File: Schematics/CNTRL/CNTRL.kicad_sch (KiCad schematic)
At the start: 129 parts, among them J1 SWD, J10 Y+, J11 Y-, J12 693071020811, J13 3.3V, J14 NAVIG I2C, J15 I2C, J16 USART, J17 PYRO1_OSTTE020104, J18 PYRO3_OSTTE020104, J19 USB_A_TE_292303-7_Horizontal, J2 CONSMA001-SMD-G-T, J20 PYRO2_OSTTE020104, J21 PYRO4_OSTTE020104, J22 Reset Jumper, J3 3S LiPo, J4 F4, J5 F3, J6 F2, J7 F1, J8 X+, J9 X-, Q1 BUK9832-55A_CUX, Q2 BUK9832-55A_CUX, Q3 BUK9832-55A_CUX, Q4 BUK9832-55A_CUX, Q5 BUK9832-55A_CUX, SW1 Omron_B3F-10xx, SW2 Omron_B3F-10xx, U1 STM32405RGT6, U2 RFM95W-915S2, U3 TPS2117DRLR, U4 TPS563200, U5 AMS1117-3.3, U7 W25Q128JVSIQ, U8 USBLC6-2SC6, Y1 12MHz_ECS-120-18-33-JGN-TR3, Y2 32.768KHz_SC32S-7PF20PPM

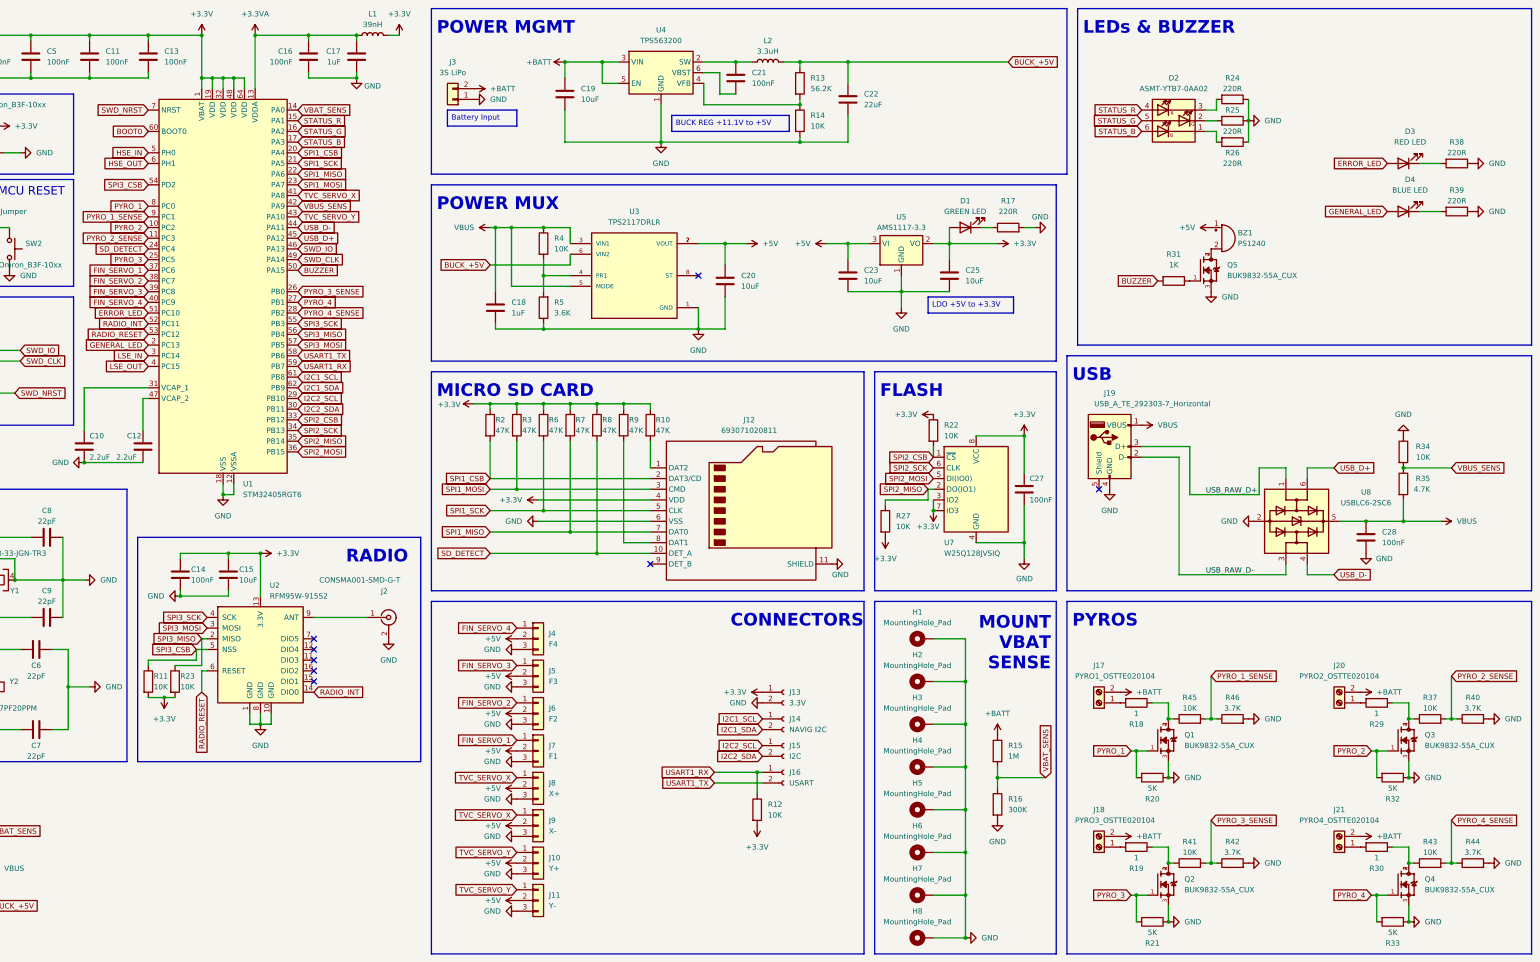
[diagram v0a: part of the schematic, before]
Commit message: CNTRL v1.1 fixes
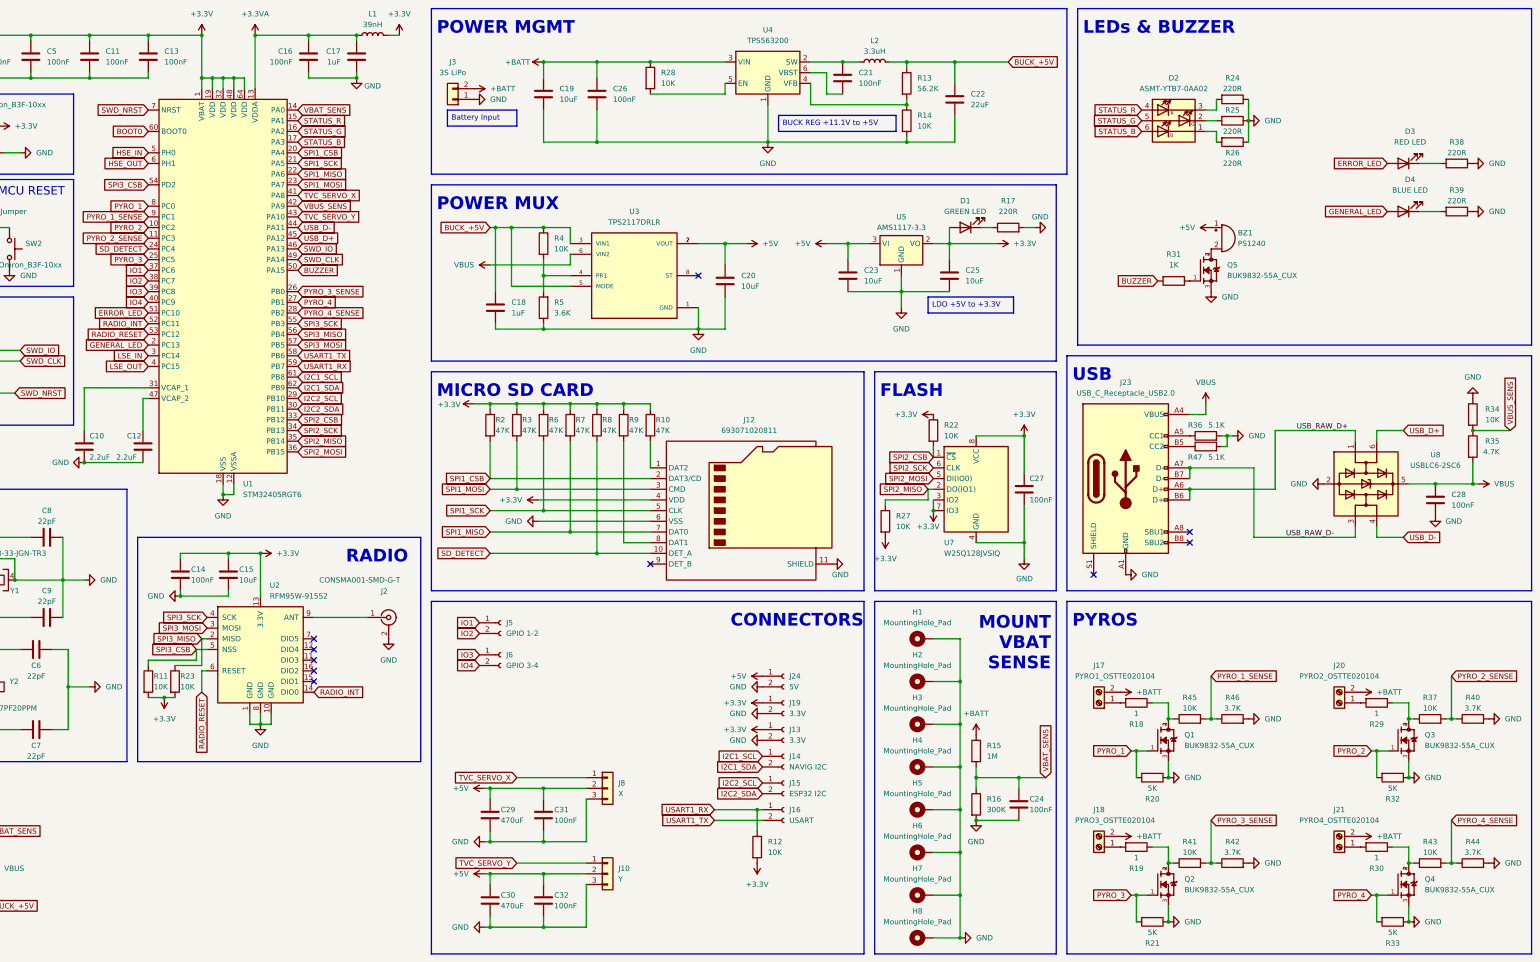
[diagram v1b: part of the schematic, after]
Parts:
- removed J11: Y-, Connector_PinHeader_2.54mm:PinHeader_1x03_P2.54mm_Vertical, symbol Connector_Generic:Conn_01x03
- removed J19: USB_A_TE_292303-7_Horizontal, Connector_USB:USB_A_TE_292303-7_Horizontal, symbol Connector:USB_A
- removed J4: F4, Connector_PinHeader_2.54mm:PinHeader_1x03_P2.54mm_Vertical, symbol Connector_Generic:Conn_01x03
- removed J5: F3, Connector_PinHeader_2.54mm:PinHeader_1x03_P2.54mm_Vertical, symbol Connector_Generic:Conn_01x03
- removed J6: F2, Connector_PinHeader_2.54mm:PinHeader_1x03_P2.54mm_Vertical, symbol Connector_Generic:Conn_01x03
- removed J7: F1, Connector_PinHeader_2.54mm:PinHeader_1x03_P2.54mm_Vertical, symbol Connector_Generic:Conn_01x03
- removed J9: X-, Connector_PinHeader_2.54mm:PinHeader_1x03_P2.54mm_Vertical, symbol Connector_Generic:Conn_01x03
- added C24, C26, C31, C32: 100nF, Capacitor_SMD:C_0603_1608Metric, symbol Device:C
- added C29, C30: 470uF, Capacitor_THT:CP_Radial_D6.3mm_P2.50mm, symbol Device:C
- added J19: 3.3V, Connector_JST:JST_XH_B2B-XH-A_1x02_P2.50mm_Vertical, symbol Connector:Conn_01x02_Socket
- added J23: USB_C_Receptacle_USB2.0, Connector_USB:USB_C_Receptacle_GCT_USB4105-xx-A_16P_TopMnt_Horizontal, symbol Connector:USB_C_Receptacle_USB2.0
- added J24: 5V, Connector_JST:JST_XH_B2B-XH-A_1x02_P2.50mm_Vertical, symbol Connector:Conn_01x02_Socket
- added J5: GPIO 1-2, TerminalBlock_Phoenix:TerminalBlock_Phoenix_MPT-0,5-2-2.54_1x02_P2.54mm_Horizontal, symbol Connector:Conn_01x02_Socket
- added J6: GPIO 3-4, TerminalBlock_Phoenix:TerminalBlock_Phoenix_MPT-0,5-2-2.54_1x02_P2.54mm_Horizontal, symbol Connector:Conn_01x02_Socket
- added R28: 10K, Resistor_SMD:R_0603_1608Metric, symbol Device:R
- added R36, R47: 5.1K, Resistor_SMD:R_0603_1608Metric, symbol Device:R
- J10: value Y+ -> Y; footprint Connector_PinHeader_2.54mm:PinHeader_1x03_P2.54mm_Vertical -> TerminalBlock_Phoenix:TerminalBlock_Phoenix_MPT-0,5-3-2.54_1x03_P2.54mm_Horizontal
- J15: value I2C -> ESP32 I2C
- J8: value X+ -> X; footprint Connector_PinHeader_2.54mm:PinHeader_1x03_P2.54mm_Vertical -> TerminalBlock_Phoenix:TerminalBlock_Phoenix_MPT-0,5-3-2.54_1x03_P2.54mm_Horizontal
- Q1, Q2, Q3, Q4, Q5: footprint BUK9832-55A_CUX:TRANS_BUK9832-55A_CUX -> External:TRANS_BUK9832-55A_CUX
- U7: footprint Package_SO:SOIC-8_5.23x5.23mm_P1.27mm -> Package_SO:SOIC-8_5.3x5.3mm_P1.27mm
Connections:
- net +3.3V: now also J19.1 (Pin_1)
- net +5V: now also C29.2, C30.2, C31.2, C32.2, J24.1 (Pin_1)
- net +BATT: now also C26.1, R28.1; no longer U4.5 (EN)
- net BUCK_+5V: now also C18.1, R4.1, U3.3 (VIN1), U3.5 (MODE); no longer U3.6 (VIN2)
- net GND: now also C24.1, C26.2, C29.1, C30.1, C31.1, C32.1, J19.2 (Pin_2), J23.A1 (GND), J23.A12 (GND), J23.B1 (GND), J23.B12 (GND), J24.2 (Pin_2), R36.2, R47.2
- net USB_RAW_D+: now also J23.A6 (D+), J23.B6 (D+)
- net USB_RAW_D-: now also J23.A7 (D-), J23.B7 (D-)
- net VBAT_SENS: now also C24.2
- net VBUS: now also U3.6 (VIN2), J23.A4 (VBUS), J23.A9 (VBUS), J23.B4 (VBUS), J23.B9 (VBUS); no longer C18.1, R4.1, U3.3 (VIN1), U3.5 (MODE)
- net FIN_SERVO_1 renamed IO1
- net IO1: now also J5.1 (Pin_1)
- net FIN_SERVO_2 renamed IO2
- net IO2: now also J5.2 (Pin_2)
- net FIN_SERVO_3 renamed IO3
- net IO3: now also J6.1 (Pin_1)
- net FIN_SERVO_4 renamed IO4
- net IO4: now also J6.2 (Pin_2)
- new net: R28.2, U4.5 (EN)
- new net: J23.B5 (CC2), R47.1
- new net: J23.A5 (CC1), R36.1
- no-connect marks 10 -> 12
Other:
- moved on the sheet: C19, C21, C22, C28, J10, J13, J14, J15, J16, J8, L2, R12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

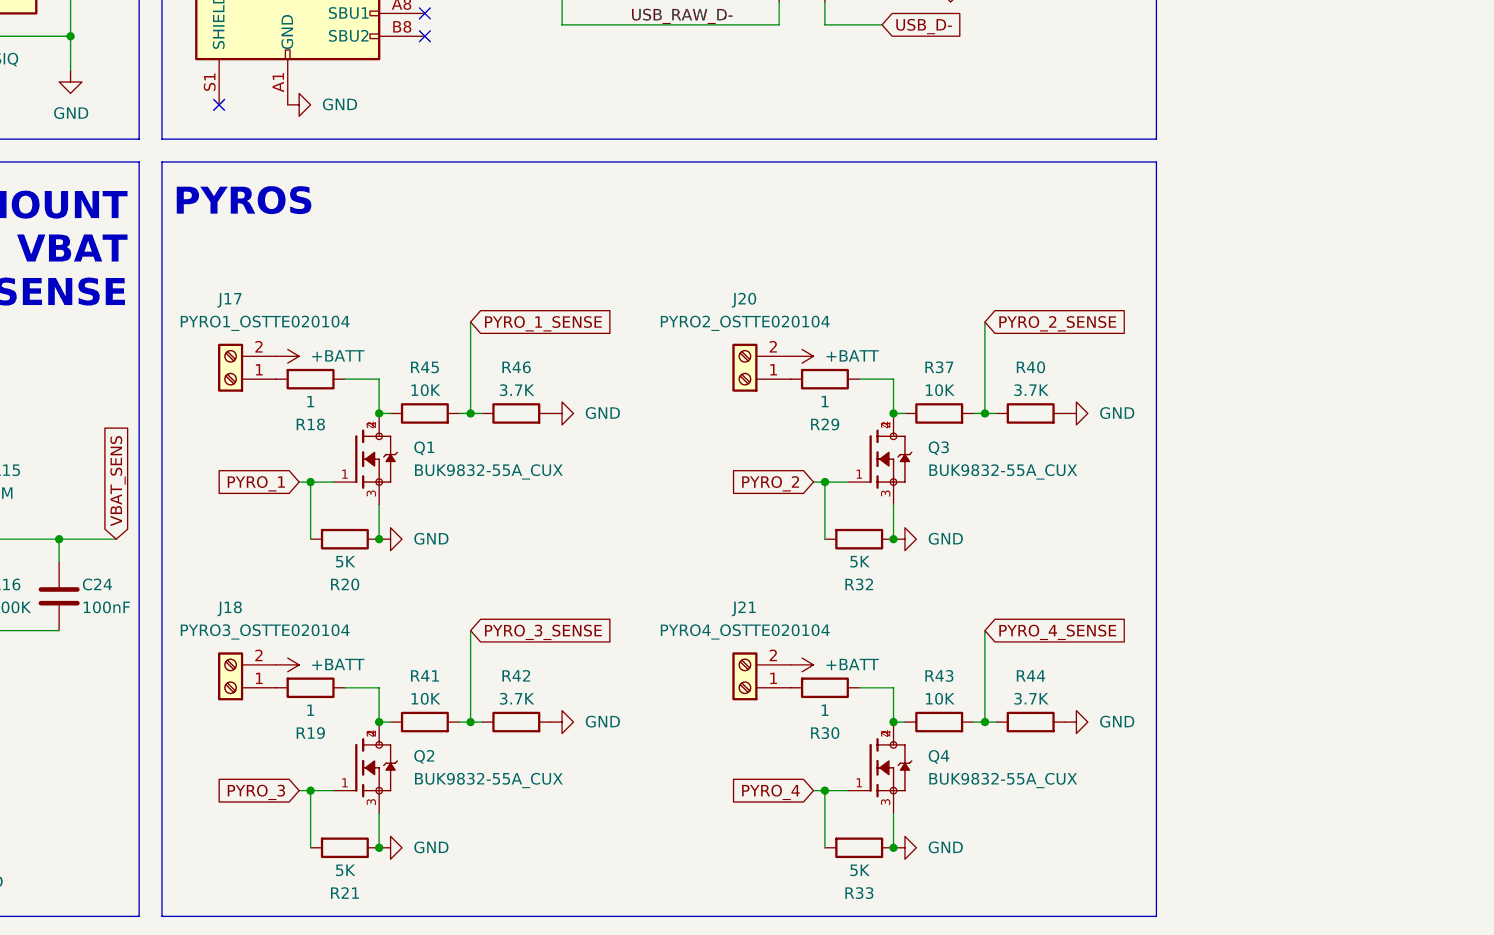
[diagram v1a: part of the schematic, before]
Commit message: final CNTRL v1.1
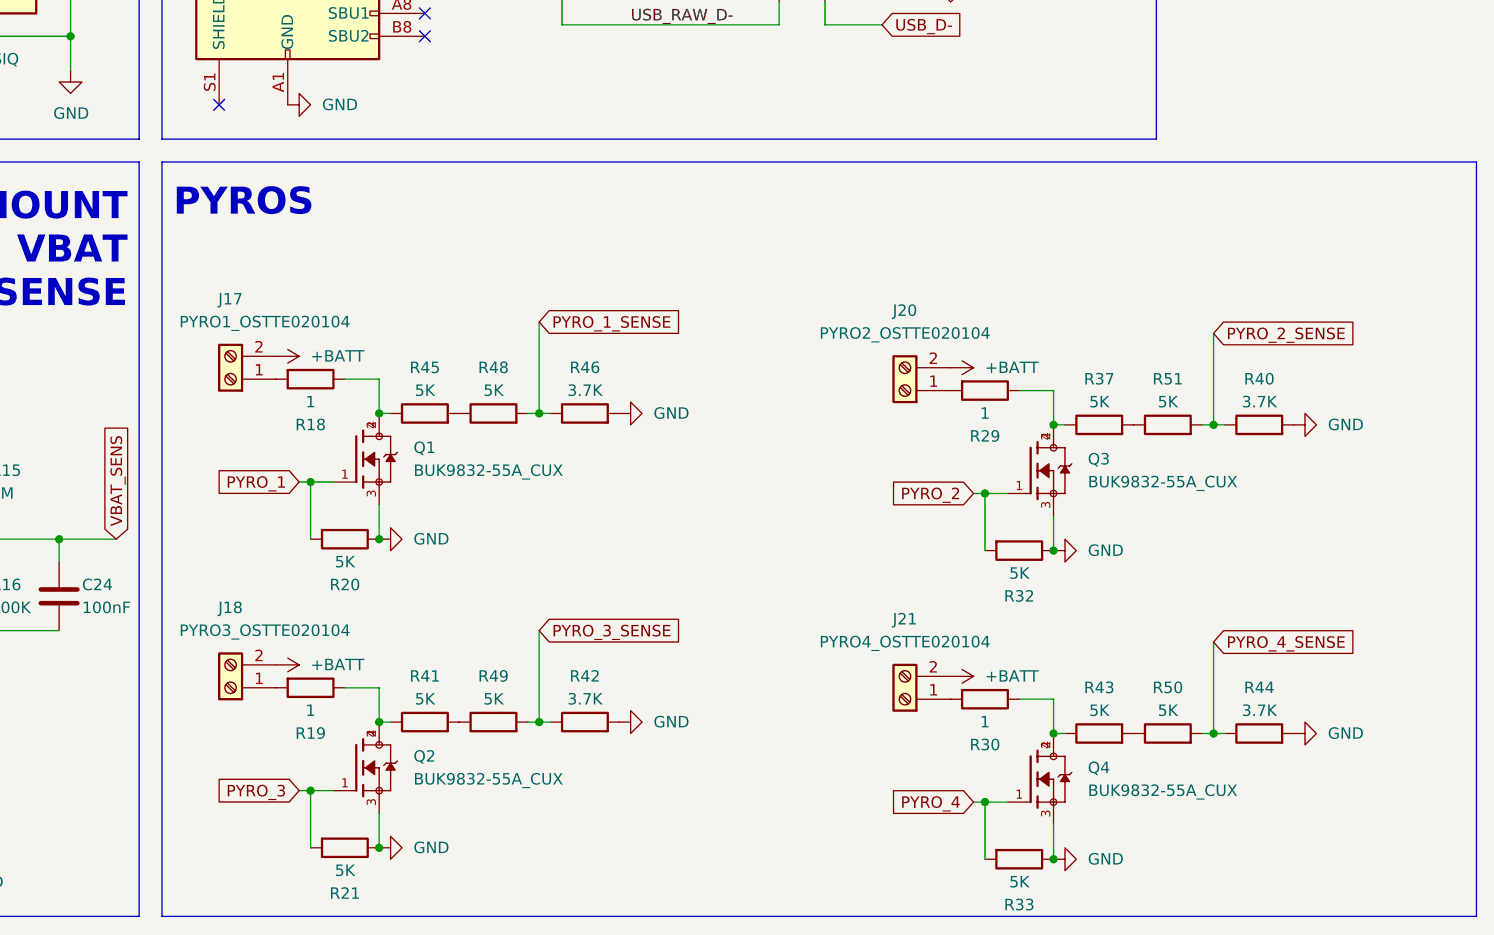
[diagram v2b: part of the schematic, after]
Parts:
- added R48, R49, R50, R51: 5K, Resistor_SMD:R_0603_1608Metric, symbol Device:R
- R37, R41, R43, R45: value 10K -> 5K
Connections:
- net PYRO_1_SENSE: now also R48.2; no longer R45.2
- net PYRO_2_SENSE: now also R51.2; no longer R37.2
- net PYRO_3_SENSE: now also R49.2; no longer R41.2
- net PYRO_4_SENSE: now also R50.2; no longer R43.2
- new net: R37.2, R51.1
- new net: R43.2, R50.1
- new net: R41.2, R49.1
- new net: R45.2, R48.1
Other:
- moved on the sheet: J20, J21, Q3, Q4, R29, R30, R32, R33, R37, R40, R42, R43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
